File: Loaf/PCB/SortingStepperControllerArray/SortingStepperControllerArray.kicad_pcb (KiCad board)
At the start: 2 copper layers, 100 x 75 mm, 34 parts, among them J1 Conn_01x04_Socket, J2 Conn_01x04_Socket, J3 Conn_01x04_Socket, J4 Conn_01x04_Socket, J5 Motor_Supply, J6 Logic_Supply, J7 Logic_Input, SW1 Limit_Switch, SW2 Limit_Switch, SW3 Limit_Switch, SW4 Limit_Switch

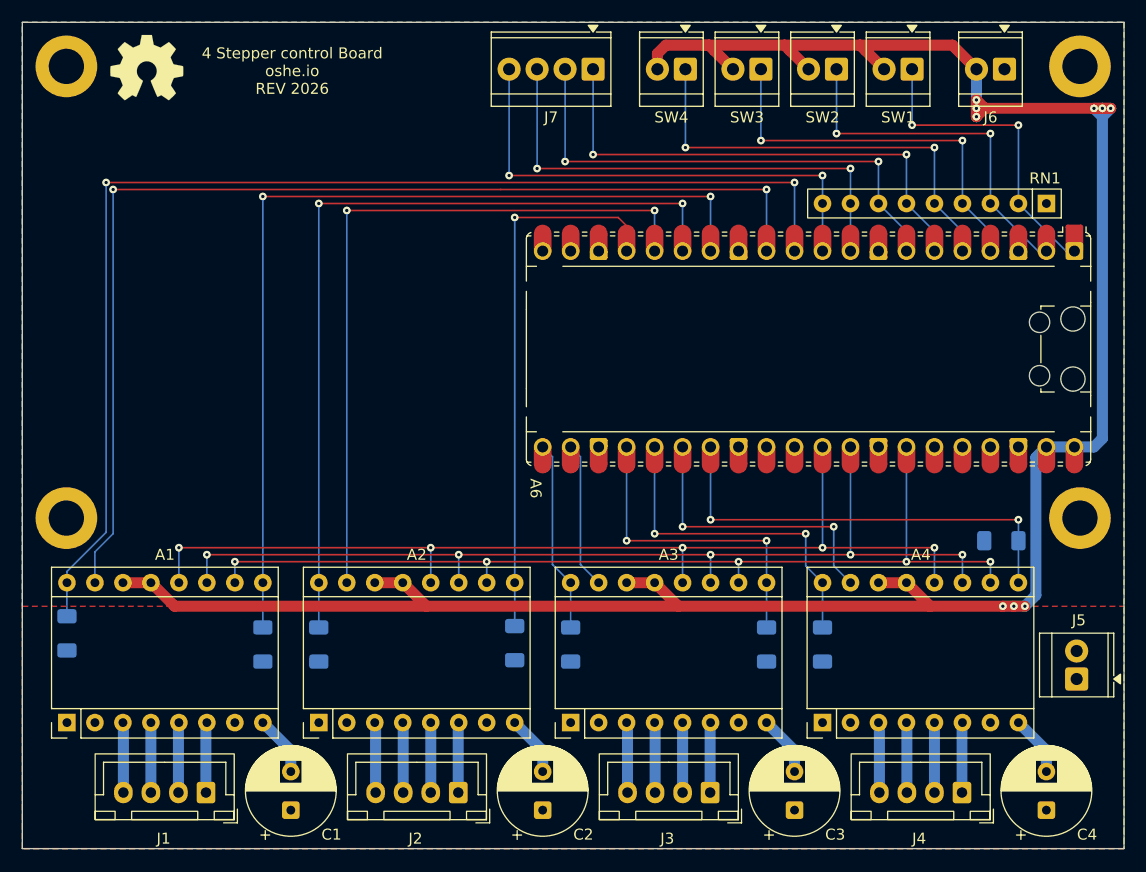
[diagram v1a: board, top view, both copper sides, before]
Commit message: Peter recommended PCB changes
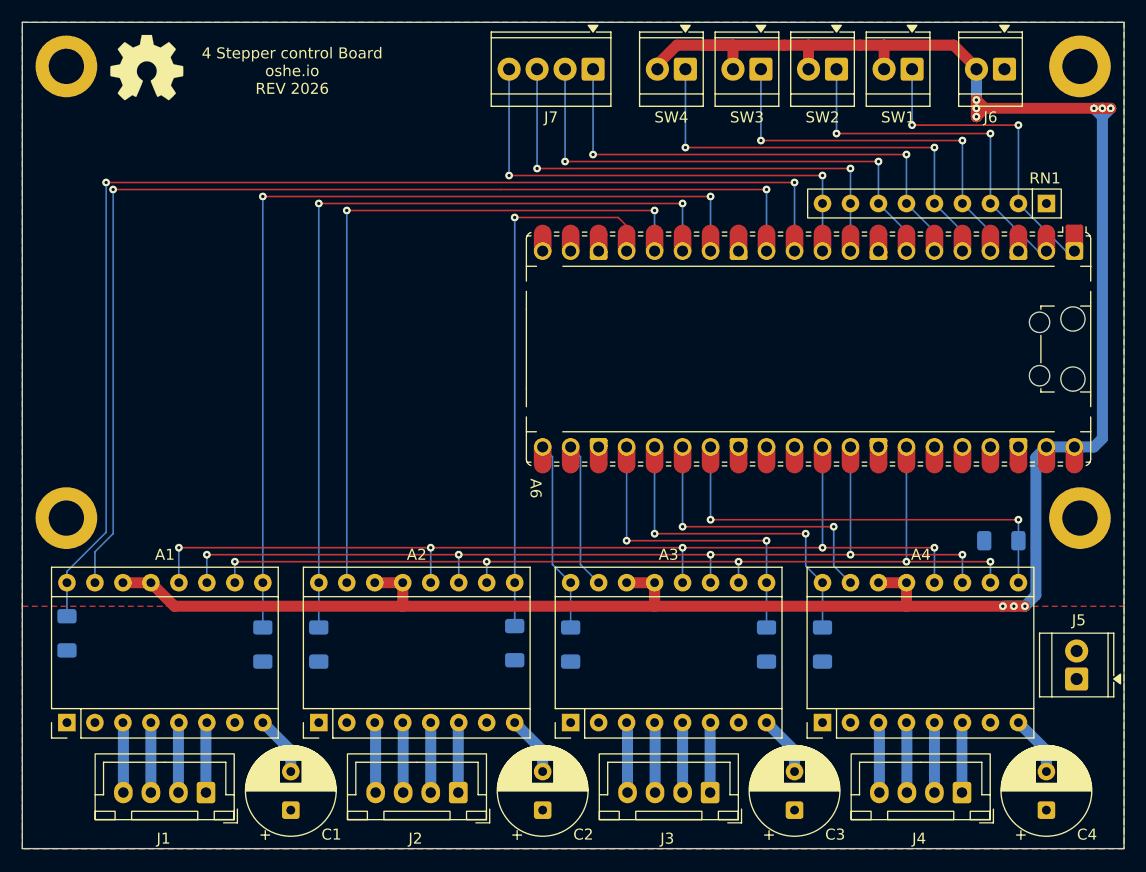
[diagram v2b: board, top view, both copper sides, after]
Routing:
- net +5V: track 221.4 -> 217.7 mm
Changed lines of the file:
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@@
 	)
 	(segment
-		(start 178.158 66.525)
-		(end 178.64 67.007)
-		(width 1)
-		(layer "F.Cu")
-		(net "+5V")
-	)
-	(segment
-		(start 143.458 115.253)
-		(end 145.658 117.453)
+		(start 180.34 66.525)
+		(end 180.34 68.707)
+		(width 1)
+		(layer "F.Cu")
+		(net "+5V")
+	)
+	(segment
+		(start 122.787 117.453)
+		(end 197.978 117.453)
+		(width 1)
+		(layer "F.Cu")
+		(net "+5V")
+	)
+	(segment
+		(start 195.585 68.585)
+		(end 195.585 68.707)
 		(width 1)
 		(layer "F.Cu")
@@
 	)
 	(segment
+		(start 193.525 66.525)
+		(end 195.585 68.585)
+		(width 1)
+		(layer "F.Cu")
+		(net "+5V")
+	)
+	(segment
+		(start 173.482 66.525)
+		(end 173.482 68.707)
+		(width 1)
+		(layer "F.Cu")
+		(net "+5V")
+	)
+	(segment
 		(start 163.83 115.316)
 		(end 166.37 115.316)
@@
 	)
 	(segment
-		(start 168.518 117.453)
-		(end 191.378 117.453)
-		(width 1)
-		(layer "F.Cu")
-		(net "+5V")
-	)
-	(segment
 		(start 197.978 117.453)
 		(end 198.978 117.453)
@@
 	)
 	(segment
-		(start 173.482 68.707)
-		(end 171.782 67.007)
+		(start 166.624 68.707)
+		(end 166.624 68.29657)
+		(width 1)
+		(layer "F.Cu")
+		(net "+5V")
+	)
+	(segment
+		(start 166.37 115.305)
+		(end 166.37 117.453)
 		(width 1)
 		(layer "F.Cu")
@@
 	)
 	(segment
-		(start 191.378 117.453)
-		(end 197.978 117.453)
-		(width 1)
-		(layer "F.Cu")
-		(net "+5V")
-	)
-	(segment
 		(start 185.016 66.525)
-		(end 193.403 66.525)
-		(width 1)
-		(layer "F.Cu")
-		(net "+5V")
-	)
-	(segment
-		(start 187.198 68.707)
-		(end 185.498 67.007)
+		(end 187.198 66.525)
 		(width 1)
 		(layer "F.Cu")
@@
 	)
 	(segment
+		(start 143.51 115.305)
+		(end 143.51 117.453)
+		(width 1)
+		(layer "F.Cu")
+		(net "+5V")
+	)
+	(segment
 		(start 198.978 117.453)
 		(end 199.978 117.453)
@@
 	)
 	(segment
-		(start 145.658 117.453)
-		(end 168.518 117.453)
-		(width 1)
-		(layer "F.Cu")
-		(net "+5V")
-	)
-	(segment
 		(start 189.178 115.253)
-		(end 191.378 117.453)
+		(end 189.23 115.305)
+		(width 1)
+		(layer "F.Cu")
+		(net "+5V")
+	)
+	(segment
+		(start 120.598 115.253)
+		(end 120.598 115.264)
 		(width 1)
 		(layer "F.Cu")
@@
 	)
 	(segment
+		(start 187.198 66.525)
+		(end 193.525 66.525)
+		(width 1)
+		(layer "F.Cu")
+		(net "+5V")
+	)
+	(segment
 		(start 195.58 73.02)
 		(end 196.337 72.263)
@@
 	)
 	(segment
-		(start 166.624 67.292787)
-		(end 167.391787 66.525)
-		(width 1)
-		(layer "F.Cu")
-		(net "+5V")
-	)
-	(segment
-		(start 166.624 68.707)
-		(end 166.624 67.292787)
-		(width 1)
-		(layer "F.Cu")
-		(net "+5V")
-	)
-	(segment
-		(start 122.798 117.453)
-		(end 145.658 117.453)
-		(width 1)
-		(layer "F.Cu")
-		(net "+5V")
-	)
-	(segment
-		(start 185.016 66.525)
-		(end 185.498 67.007)
+		(start 189.23 115.305)
+		(end 189.23 117.453)
+		(width 1)
+		(layer "F.Cu")
+		(net "+5V")
+	)
+	(segment
+		(start 187.198 66.525)
+		(end 187.198 68.707)
+		(width 1)
+		(layer "F.Cu")
+		(net "+5V")
+	)
+	(segment
+		(start 166.624 68.29657)
+		(end 168.39557 66.525)
+		(width 1)
+		(layer "F.Cu")
+		(net "+5V")
+	)
+	(segment
+		(start 168.39557 66.525)
+		(end 173.482 66.525)
 		(width 1)
 		(layer "F.Cu")
@@
 	)
 	(segment
-		(start 171.3 66.525)
-		(end 171.782 67.007)
+		(start 166.318 115.253)
+		(end 166.37 115.305)
 		(width 1)
 		(layer "F.Cu")
@@
 	(segment
 		(start 178.158 66.525)
-		(end 185.016 66.525)
-		(width 1)
-		(layer "F.Cu")
-		(net "+5V")
-	)
-	(segment
-		(start 166.318 115.253)
-		(end 168.518 117.453)
+		(end 180.34 66.525)
 		(width 1)
 		(layer "F.Cu")
@@
 	)
 	(segment
-		(start 120.598 115.253)
-		(end 122.798 117.453)
+		(start 180.34 66.525)
+		(end 185.016 66.525)
+		(width 1)
+		(layer "F.Cu")
+		(net "+5V")
+	)
+	(segment
+		(start 120.598 115.264)
+		(end 122.787 117.453)
 		(width 1)
 		(layer "F.Cu")
@@
 	)
 	(segment
+		(start 143.458 115.253)
+		(end 143.51 115.305)
+		(width 1)
+		(layer "F.Cu")
+		(net "+5V")
+	)
+	(segment
 		(start 196.337 72.263)
 		(end 196.337 72.258)
 		(width 1)
 		(layer "F.Cu")
-		(net "+5V")
-	)
-	(segment
-		(start 167.391787 66.525)
-		(end 171.3 66.525)
-		(width 1)
-		(layer "F.Cu")
-		(net "+5V")
-	)
-	(segment
-		(start 193.403 66.525)
-		(end 195.585 68.707)
-		(width 1)
-		(layer "F.Cu")
-		(net "+5V")
-	)
-	(segment
-		(start 180.34 68.707)
-		(end 178.64 67.007)
-		(width 1)
-		(layer "F.Cu")
